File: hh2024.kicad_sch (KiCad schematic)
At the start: 60 parts, among them J1 SAO, J2 QWIIC, J3 Micro_SD_Card, J4 USB-C, J7 RELAY, J9 CH32Prog, K1 SANYOU_SRD_Form_C, Q3 AP2302B, SW1 Multi-Directional-Switches, SW2 Multi-Directional-Switches, SW3 Multi-Directional-Switches, SW4 Multi-Directional-Switches, SW5 Multi-Directional-Switches, U5 CH32V003F4U6, U6 74LVC1G125

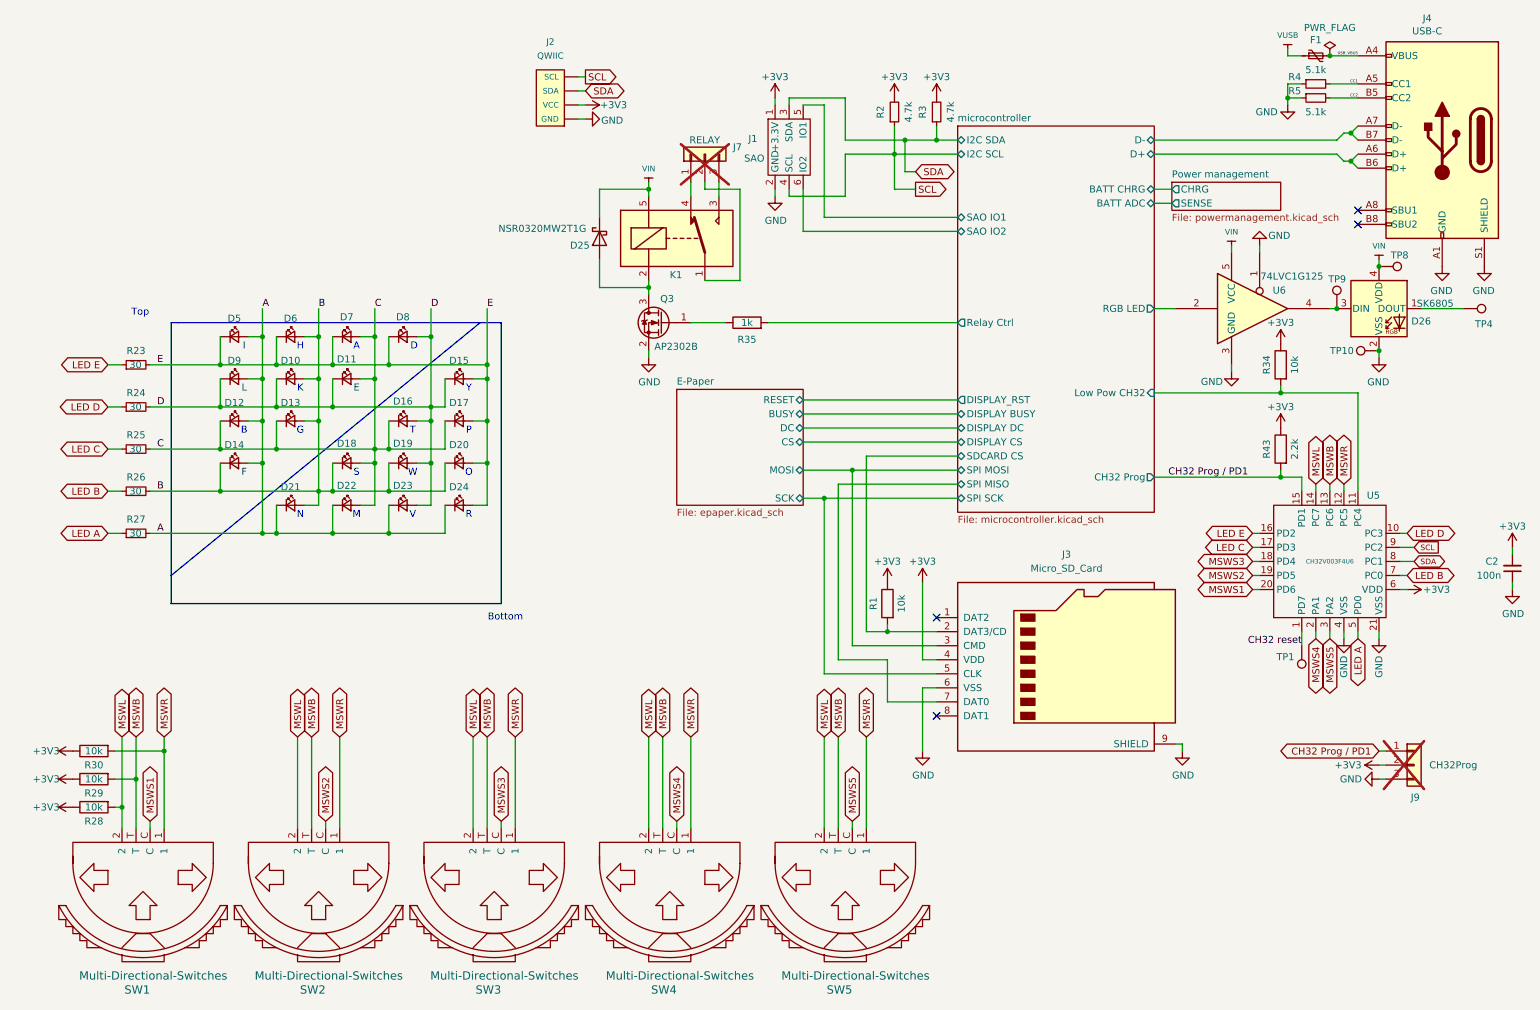
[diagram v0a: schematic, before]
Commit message: Moar headers
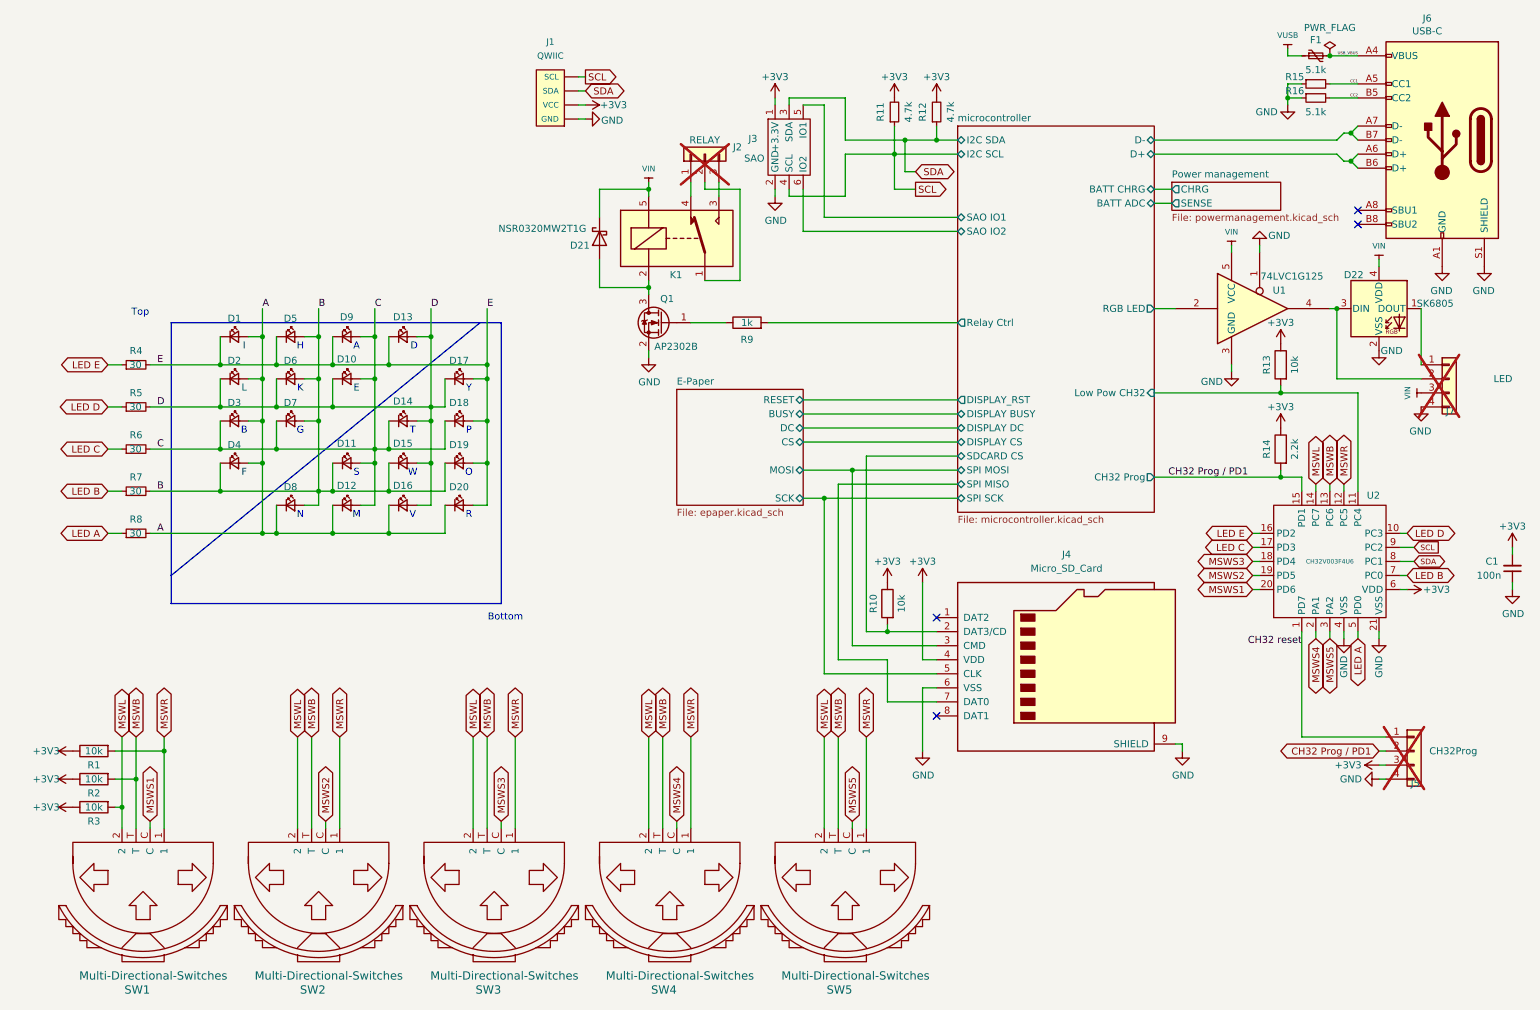
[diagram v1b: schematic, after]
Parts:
- removed TP1, TP10, TP4, TP8, TP9: TestPoint, TestPoint:TestPoint_Pad_1.0x1.0mm, symbol Connector:TestPoint
- added J7: LED, Connector_PinHeader_2.54mm:PinHeader_1x04_P2.54mm_Vertical, symbol Connector_Generic:Conn_01x04
- J5: renamed from J9; footprint Connector_PinHeader_2.54mm:PinHeader_1x03_P2.54mm_Vertical -> Connector_PinHeader_2.54mm:PinHeader_2x02_P2.54mm_Vertical; symbol Connector_Generic:Conn_01x03 -> Connector_Generic:Conn_01x04; now in the parts list
- renumbered C2 to C1, D5 to D1, D11 to D10, D18 to D11, D22 to D12, D8 to D13, D16 to D14, D19 to D15, D23 to D16, D15 to D17, D17 to D18, D20 to D19, D9 to D2, D24 to D20, D25 to D21, D26 to D22, D12 to D3, D14 to D4, D6 to D5, D10 to D6, D13 to D7, D21 to D8, D7 to D9, J2 to J1, J7 to J2, J1 to J3, J3 to J4, J4 to J6, Q3 to Q1, R30 to R1, R1 to R10, R2 to R11, R3 to R12, R34 to R13, R43 to R14, R4 to R15, R5 to R16, R29 to R2, R28 to R3, R23 to R4, R24 to R5, R25 to R6, R26 to R7, R27 to R8, R35 to R9, U6 to U1, U5 to U2
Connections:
- net +3V3: now also J5.3 (Pin_3); no longer J5.2 (Pin_2)
- net CH32 Prog / PD1: now also J5.2 (Pin_2); no longer J5.1 (Pin_1)
- net CH32 reset: now also J5.1 (Pin_1)
- net GND: now also J5.4 (Pin_4), J7.4 (Pin_4); no longer J5.3 (Pin_3)
- net VIN: now also J7.3 (Pin_3)
- net at D22.1 (DOUT): now also J7.1 (Pin_1)
- net at D22.3 (DIN), U1.4: now also J7.2 (Pin_2)
